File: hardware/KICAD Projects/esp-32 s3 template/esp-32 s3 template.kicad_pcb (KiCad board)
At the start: 2 copper layers, 62.5 x 32.5 mm, 39 parts, among them J1 TYPE-C-31-M-12, J2 DTF13-6P, SW1 PTS810_SJM_250_SMTR_LFS, SW2 PTS810_SJM_250_SMTR_LFS, U1 AMS1117-3.3, U2 ESP32-S3-WROOM-1, U3 MCP2515-I, U4 TJA1050DRG, X1 8MHz

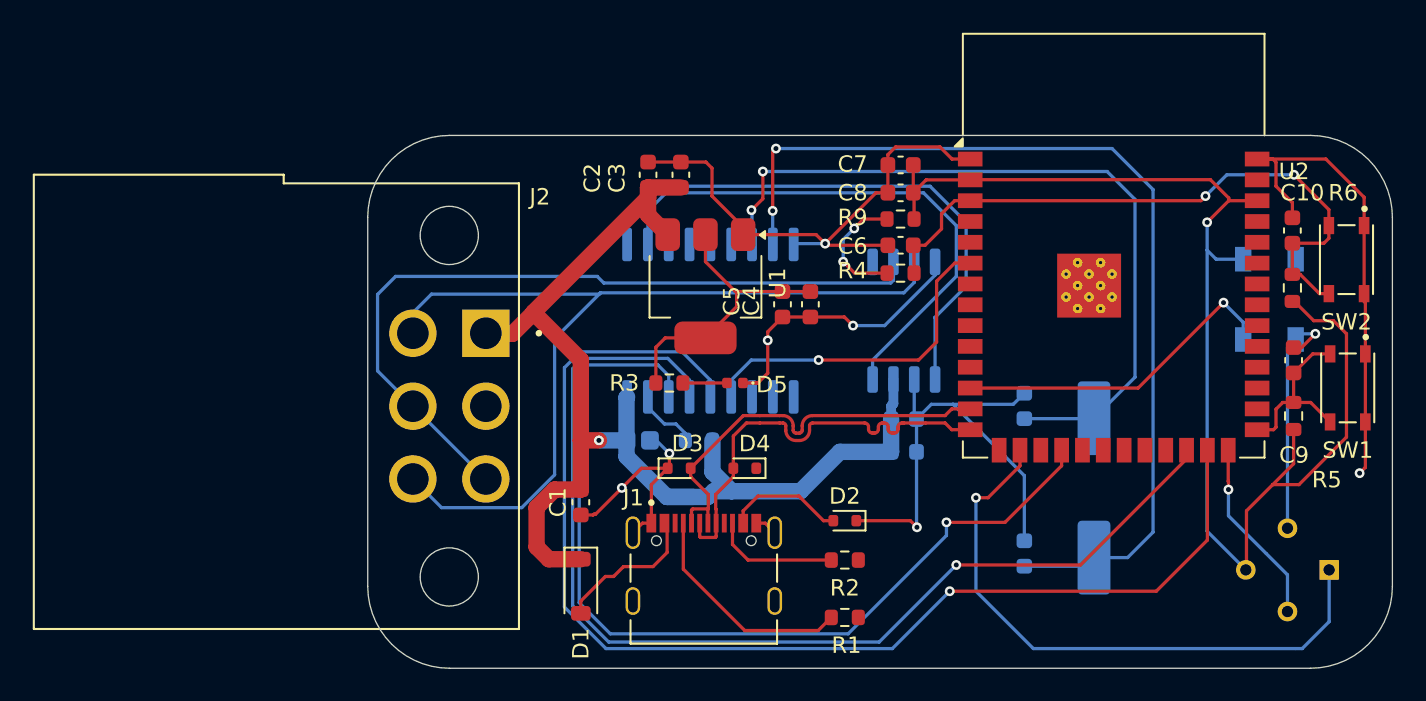
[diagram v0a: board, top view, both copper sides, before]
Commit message: Finished it
Figured out zone fills
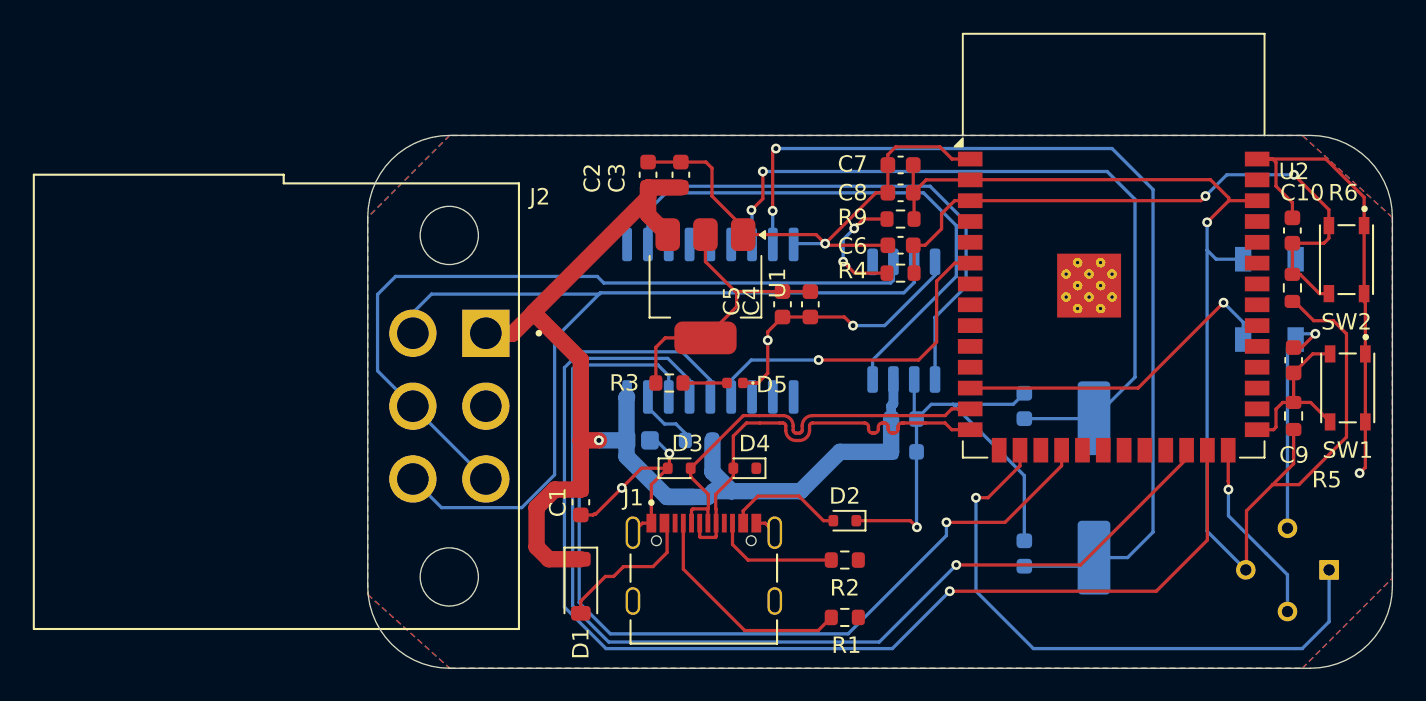
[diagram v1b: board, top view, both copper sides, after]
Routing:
- added copper zone on B.Cu, net GND
- added copper zone on F.Cu, net GND
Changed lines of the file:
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@@
 		(net 58)
+	)
+	(zone
+		(net 2)
+		(net_name "GND")
+		(layers "F.Cu" "B.Cu")
+		(hatch edge 0.5)
+		(connect_pads
+			(clearance 0.5)
+		)
+		(min_thickness 0.25)
+		(filled_areas_thickness no)
+		(fill yes
+			(thermal_gap 0.5)
+			(thermal_bridge_width 0.5)
+		)
+		(polygon
+			(pts
+				(xy 110 35) (xy 105 40) (xy 105 63) (xy 110 67.5) (xy 162 67.5) (xy 167.5 62) (xy 167.5 40) (xy 162 35)
+			)
+		)
 	)
 	(generated
